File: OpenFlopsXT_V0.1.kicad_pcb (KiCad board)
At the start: 2 copper layers, 83.9 x 68.6 mm, 77 parts, among them J1 UP, J2 DN, J3 R, J4 G, J5 FH12-24S-0.5SH(55), J6 OSHW_LOGO, P1 FLOPPY_CONN, P2 POWER_INPUT, P3 POWER_PASSTHRU, P4 PROG_PORT, P6 ENCODER_PORT, P7 DISPLAY_PORT, P8 USB_HEADER, P9 SPK, Q1 BSS138, Q2 BSS138, Q3 BSS138, Q4 BSS138, Q5 BSS138, Q6 BSS138, Q7 MMBT3904, U1 74HCT04, U3 STM32F105RBT6, U4 LM1117-3.3, Y1 8 MHz

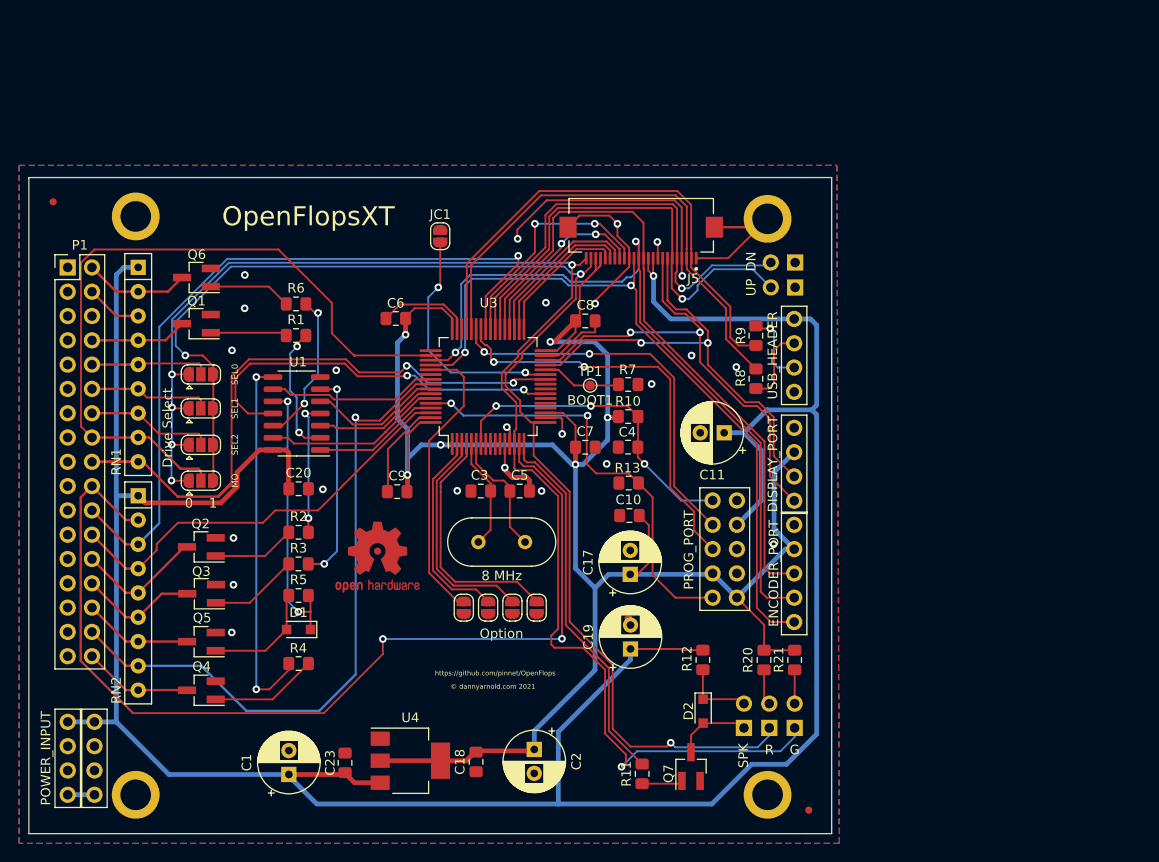
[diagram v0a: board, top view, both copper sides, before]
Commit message: Added 3d images of OpenFlopsXT
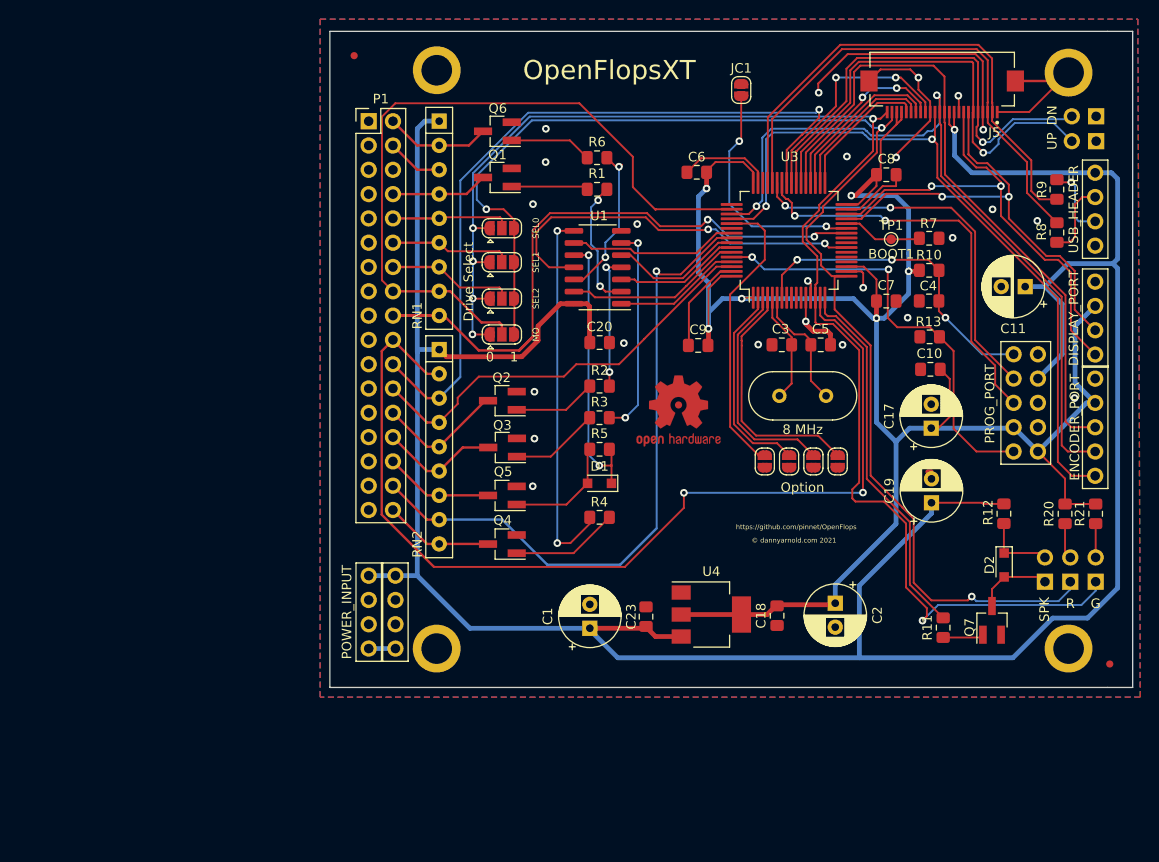
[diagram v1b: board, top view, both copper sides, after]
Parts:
- moved FID2 35.0 mm to (189.2, 127.0)
- moved C10 35.0 mm to (170.4, 96.2)
- moved C17 35.0 mm to (170.5, 102.4)
- moved C19 35.0 mm to (170.6, 110.2)
- moved H2 35.0 mm to (184.9, 125.4)
- moved J5 35.0 mm to (171.7, 66.6)
- moved JP5 35.0 mm to (153.1, 105.9)
- moved P6 35.0 mm to (187.7, 97.2)
- moved P8 35.0 mm to (187.7, 75.7)
- moved Q7 35.0 mm to (176.9, 122.5)
- moved R10 35.0 mm to (170.3, 85.9)
- moved R11 35.0 mm to (171.8, 123.2)
- moved R7 35.0 mm to (170.3, 82.5)
- moved R8 35.0 mm to (183.7, 81.9)
- moved R9 35.0 mm to (183.7, 77.4)
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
